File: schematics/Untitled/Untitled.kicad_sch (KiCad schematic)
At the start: 27 parts, among them M1 Motor_DC, Q1 NPN, Q2 PNP, Q3 NPN, Q4 NPN, Q5 NPN, Q6 NPN, U1 INA260, U2 XL1509-3.3

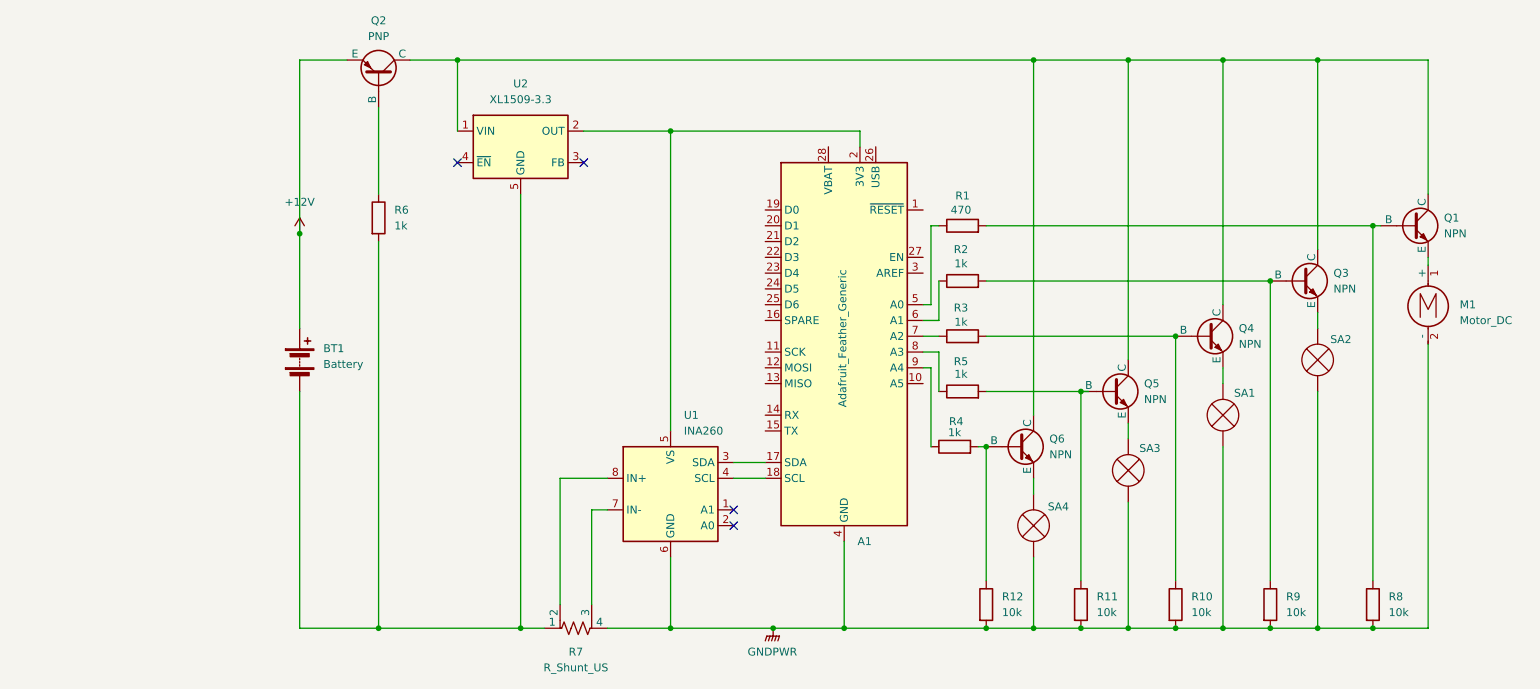
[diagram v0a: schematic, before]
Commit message: One Big Mess
Just a lot of updates
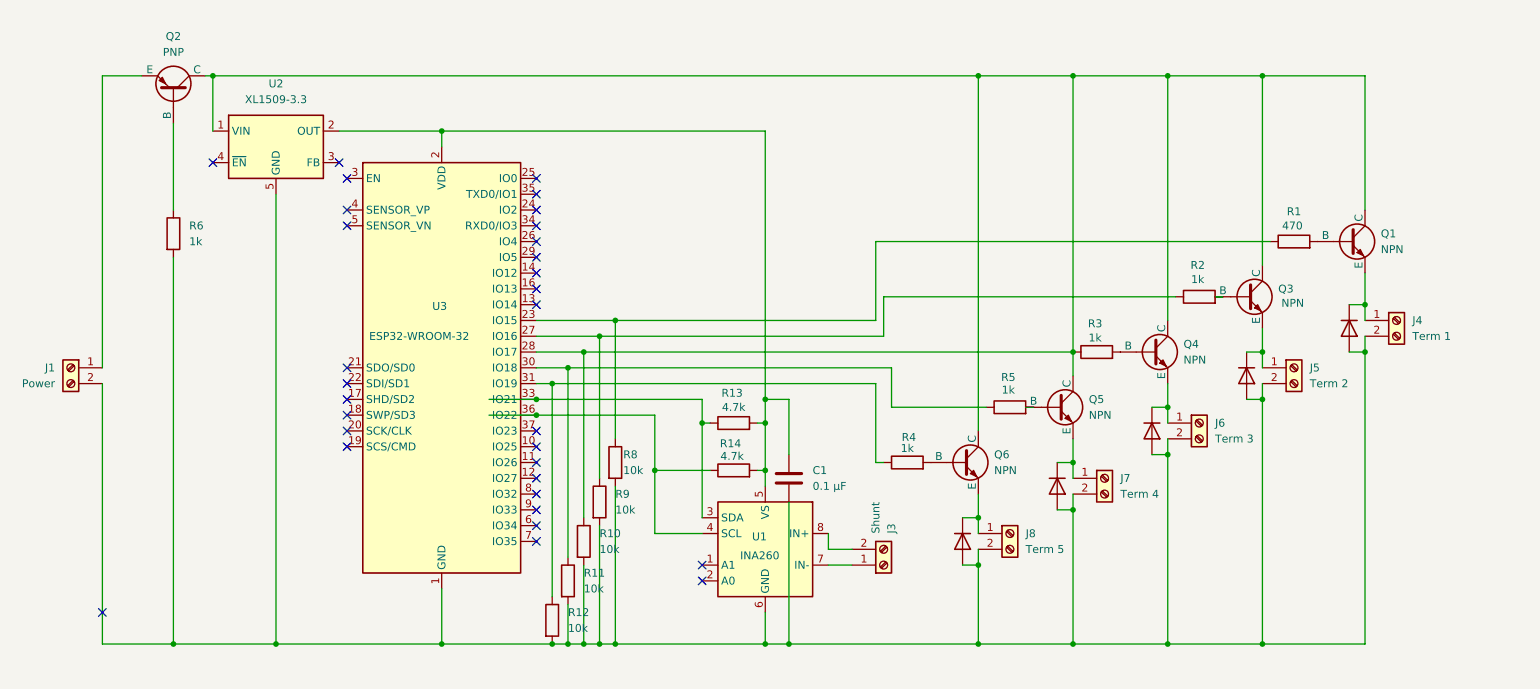
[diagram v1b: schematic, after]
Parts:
- removed A1: Adafruit_Feather_Generic, Module:Adafruit_Feather, symbol MCU_Module:Adafruit_Feather_Generic
- removed BT1: Battery, symbol Device:Battery
- removed M1: Motor_DC, symbol Motor:Motor_DC
- removed R7: R_Shunt_US, symbol Device:R_Shunt_US
- removed SA1, SA2, SA3, SA4: Solenoid, symbol Device:Lamp
- added C1: 0.1 µF, Resistor_THT:R_Axial_DIN0207_L6.3mm_D2.5mm_P7.62mm_Horizontal, symbol Device:C
- added D1, D2, D3, D4, D5: D, Resistor_THT:R_Axial_DIN0207_L6.3mm_D2.5mm_P7.62mm_Horizontal, symbol Device:D
- added J1: Power, TerminalBlock:TerminalBlock_Altech_AK300-2_P5.00mm, symbol Connector:Screw_Terminal_01x02
- added J3: Shunt, TerminalBlock:TerminalBlock_Altech_AK300-2_P5.00mm, symbol Connector:Screw_Terminal_01x02
- added J4: Term 1, TerminalBlock:TerminalBlock_Altech_AK300-2_P5.00mm, symbol Connector:Screw_Terminal_01x02
- added J5: Term 2, TerminalBlock:TerminalBlock_Altech_AK300-2_P5.00mm, symbol Connector:Screw_Terminal_01x02
- added J6: Term 3, TerminalBlock:TerminalBlock_Altech_AK300-2_P5.00mm, symbol Connector:Screw_Terminal_01x02
- added J7: Term 4, TerminalBlock:TerminalBlock_Altech_AK300-2_P5.00mm, symbol Connector:Screw_Terminal_01x02
- added J8: Term 5, TerminalBlock:TerminalBlock_Altech_AK300-2_P5.00mm, symbol Connector:Screw_Terminal_01x02
- added R13, R14: 4.7k, Resistor_THT:R_Axial_DIN0207_L6.3mm_D2.5mm_P7.62mm_Horizontal, symbol Device:R
- added U3: ESP32-WROOM-32, RF_Module:ESP32-WROOM-32, symbol RF_Module:ESP32-WROOM-32
- Q1, Q2, Q3, Q4, Q5, Q6: footprint (none) -> Package_TO_SOT_THT:TO-220-3_Vertical
- R1, R10, R11, R12, R2, R3, R4, R5, R6, R8, R9: footprint (none) -> Resistor_THT:R_Axial_DIN0207_L6.3mm_D2.5mm_P7.62mm_Horizontal
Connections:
- net GNDPWR is gone; now on an unnamed net: R10.2, R11.2, R12.2, R8.2, R9.2, U1.6 (GND)
- net at Q1.1 (C), Q2.1 (C), Q3.1 (C)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: now also R10.1, R3.1, U3.28 (IO17)
- net at Q5.2 (B), R5.2: no longer R11.1
- net at Q5.3 (E): now also D4.1 (K), J7.1 (Pin_1)
- net at R2.1: now also R9.1, U3.27 (IO16)
- net at Q3.2 (B), R2.2: no longer R9.1
- net at Q3.3 (E): now also D2.1 (K), J5.1 (Pin_1)
- net at Q1.2 (B), R1.2: no longer R8.1
- net at Q1.3 (E): now also D1.1 (K), J4.1 (Pin_1)
- net at U1.5 (VS), U2.2 (OUT): now also C1.1, R13.2, R14.2, U3.2 (VDD)
- net at R6.2, U2.5 (GND), U2.6 (GND)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: now also C1.2, D1.2 (A), D2.2 (A), D3.2 (A), D4.2 (A), D5.2 (A), J1.2 (Pin_2), J4.2 (Pin_2), J5.2 (Pin_2), J6.2 (Pin_2), J7.2 (Pin_2), J8.2 (Pin_2), U3.1 (GND), U3.15 (GND), U3.38 (GND), U3.39 (GND)
- net at U1.8 (IN+): now also J3.2 (Pin_2)
- net at U1.7 (IN-): now also J3.1 (Pin_1)
- net at Q4.2 (B), R3.2: no longer R10.1
- net at Q4.3 (E): now also D3.1 (K), J6.1 (Pin_1)
- net at Q6.2 (B), R4.2: no longer R12.1
- net at U1.3 (SDA): now also R13.1, U3.33 (IO21)
- net at U1.4 (SCL): now also R14.1, U3.36 (IO22)
- net at R1.1: now also R8.1, U3.23 (IO15)
- net at R5.1: now also R11.1, U3.30 (IO18)
- net at R4.1: now also R12.1, U3.31 (IO19)
- net at Q6.3 (E): now also D5.1 (K), J8.1 (Pin_1)
- net +12V: no longer names the net of Q2.3 (E)
- net +12V: now also J1.1 (Pin_1)
- no-connect marks 4 -> 31
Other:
- moved on the sheet: Q1, Q2, Q3, Q4, Q5, Q6, R1, R10, R11, R12, R2, R3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
